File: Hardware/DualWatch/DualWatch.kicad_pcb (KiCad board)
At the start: 4 copper layers, 41.2 x 42.1 mm, 154 parts, among them J1 NFC, J2 NRF_Debug, J3 USB_C_Receptacle_USB2.0, J4 Conn_01x02_Pin, Q1 BSS123, Q2 IRLM2803, U1 NRF5340-QKAA-R7, U10 SN74LV1T34DCK, U11 SN74LV1T34DCK, U12 SN74LV1T34DCK, U13 SN74LV1T34DCK, U14 SN74LV1T34DCK, U15 SN74LV1T34DCK, U16 SN74LV1T34DCK, U17 SN74LV1T34DCK, U18 SN74LV1T34DCK, U20 NPM1100-QDAA-R7, U21 TPS63030DSK, U22 TPS63030DSK, U23 SN74LV1T34DCK, U24 SN74LV1T34DCK, U3 74LVC1G3157, U4 NRF7002-QFAA-R, U5 DPX165950DT-8126A1, U7 LIS3DH, U8 SN74LV1T34DCK, Y1 32.768kHz, Y2 32MHz, Y3 40Mhz

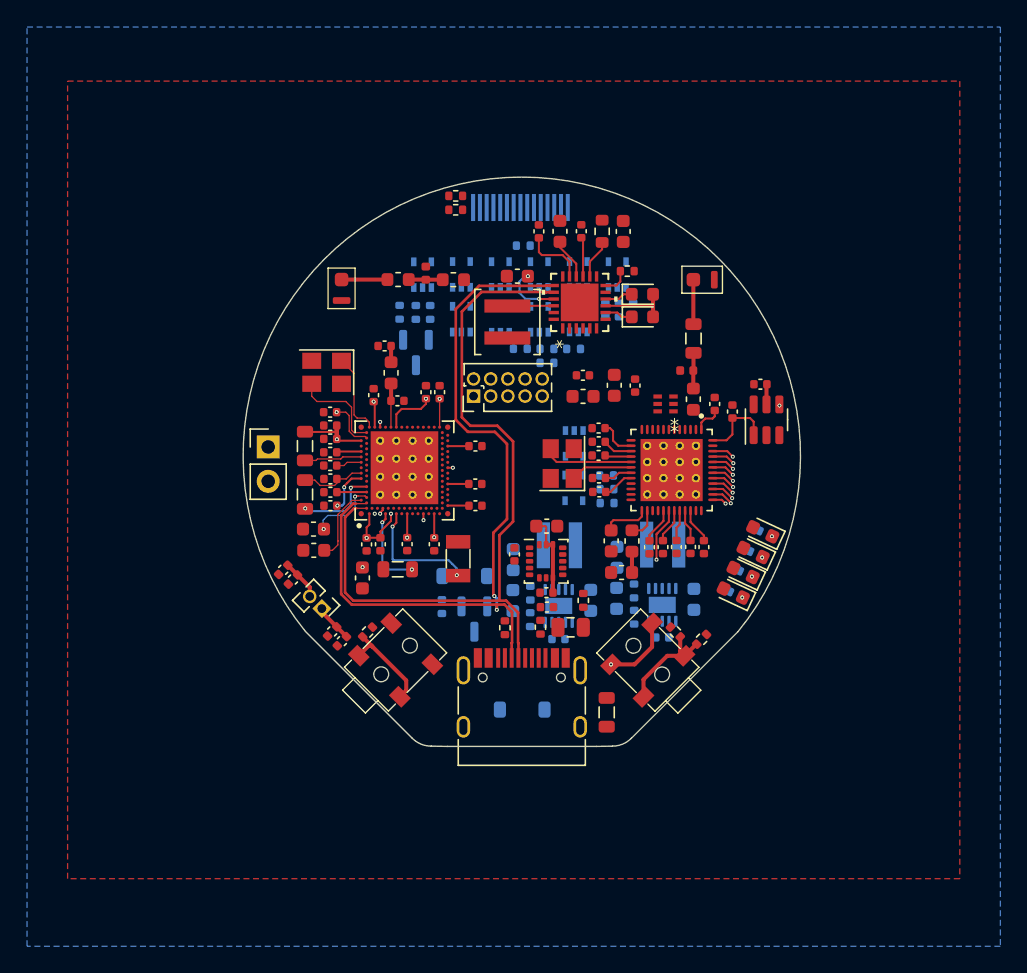
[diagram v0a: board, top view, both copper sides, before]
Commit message: update pcb
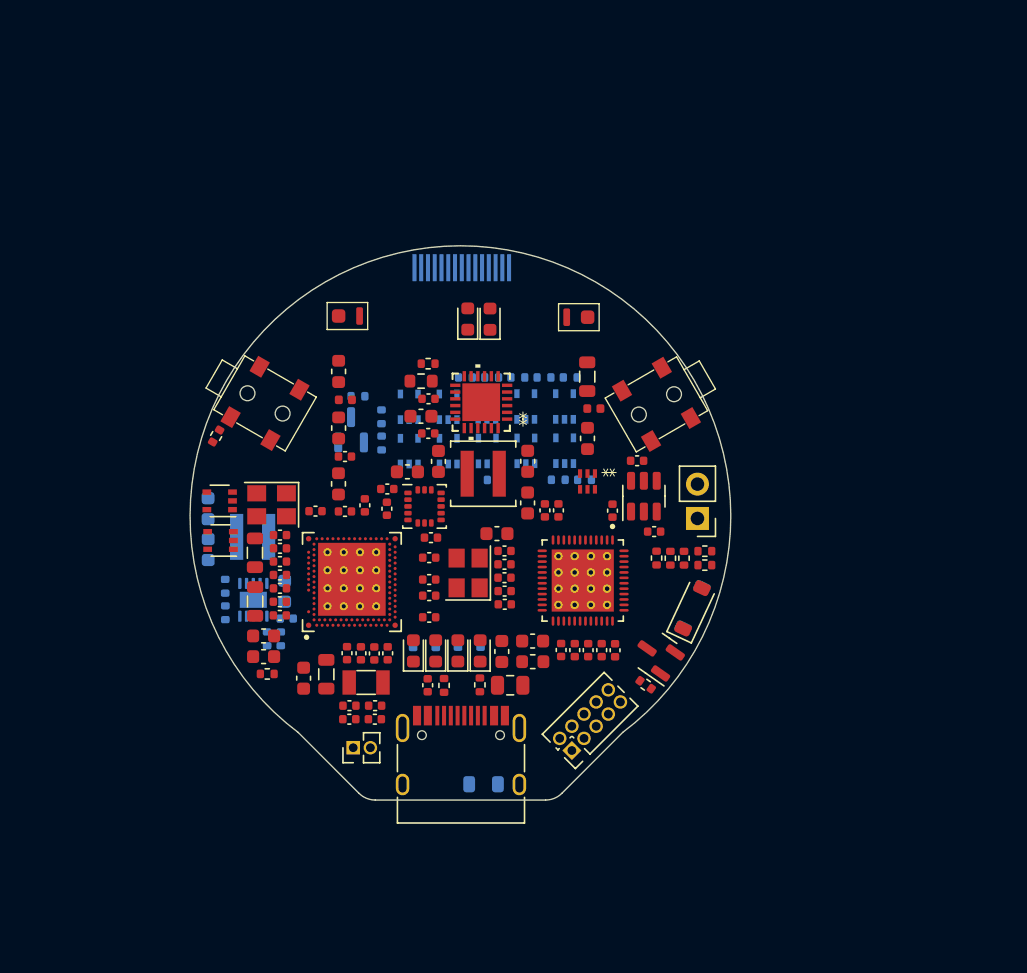
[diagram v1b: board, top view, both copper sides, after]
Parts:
- removed C60, C61, C62, C63: 10uF, Capacitor_SMD:C_0603_1608Metric
- removed L15: 1.5uH, Inductor_SMD:L_Coilcraft_XAL4020-XXX
- removed R31: 100R, Resistor_SMD:R_0402_1005Metric
- removed R32: 10K, Resistor_SMD:R_0402_1005Metric
- removed U23, U24: SN74LV1T34DCK, Package_TO_SOT_SMD:SOT-353_SC-70-5
- added U9: SN74LV1T34DCK, Package_TO_SOT_SMD:SOT-353_SC-70-5, B.Cu at (139.2, 90.4)
- C59: value 100nF -> 10uF; footprint Capacitor_SMD:C_0402_1005Metric -> Capacitor_SMD:C_0603_1608Metric
- D4, Q2, R18: moved to F.Cu
- L8: moved to B.Cu
- R21: value 100K -> 178K
- R22: value 178K -> 1M
- R23: value 261K -> 1K; moved to F.Cu
- R24: value 1M -> 10K; moved to F.Cu
- R25: value 1K -> 10K
- R26: value 10K -> 100R; moved to B.Cu
- R27: value 10K -> 100R
- R30: value 100R -> 10K; moved to F.Cu
- U18: value SN74LV1T34DCK -> ~; footprint Package_TO_SOT_SMD:SOT-353_SC-70-5 -> 1-28-LCD-Touch:1.28LCD-TP
- U19: value ~ -> NPM1100-QDAA-R7; footprint 1-28-LCD-Touch:1.28LCD-TP -> NPM1100-QDAA-R7:QFN24_NPM1100_NOR; moved to F.Cu
- U20: value NPM1100-QDAA-R7 -> TPS63030DSK; footprint NPM1100-QDAA-R7:QFN24_NPM1100_NOR -> Package_SON:WSON-10-1EP_2.5x2.5mm_P0.5mm_EP1.2x2mm; moved to B.Cu
- U21, U22: value TPS63030DSK -> SN74LV1T34DCK; footprint Package_SON:WSON-10-1EP_2.5x2.5mm_P0.5mm_EP1.2x2mm -> Package_TO_SOT_SMD:SOT-353_SC-70-5; moved to F.Cu
- moved R30 40.5 mm to (122.0, 89.3), turned to 60 degrees
- moved C58 36.1 mm to (121.4, 97.7)
- moved C59 34.9 mm to (121.4, 94.6), turned to 90 degrees
- moved U22 33.6 mm to (122.2, 94.1), turned to 180 degrees
- moved U20 32.7 mm to (124.7, 101.4), turned to -90 degrees
- moved J4 32.2 mm to (157.6, 95.4), turned to 180 degrees
- moved R15 32.1 mm to (158.1, 97.8), turned to 0 degrees
- moved R16 32.1 mm to (158.1, 98.8), turned to 180 degrees
- moved R22 30.3 mm to (122.7, 100.4)
- moved R19 27.5 mm to (125.8, 104.3), turned to 90 degrees
- moved D5 27.3 mm to (136.6, 105.1), turned to 90 degrees
- moved J2 27.2 mm to (148.3, 112.5), turned to 135 degrees
- moved R20 27.0 mm to (126.8, 104.3), turned to -90 degrees
- moved R29 26.4 mm to (136.6, 105.4), turned to 90 degrees
- moved U21 25.5 mm to (122.3, 97.0), turned to 180 degrees
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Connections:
- C54 pad 2: Net-(U20-DEC) -> Net-(U19-DEC)
- C57 pad 2: Net-(U21-PS/SYNC) -> Net-(U20-PS/SYNC)
- C58 pad 1: VIN -> +3V3
- C59 pad 1: GND -> +3V3
- C59 pad 2: Net-(U22-PS/SYNC) -> GND
- L13 pad 1: Net-(U20-SW) -> Net-(U19-SW)
- L14 pad 1: Net-(U21-L2) -> Net-(U20-L2)
- L14 pad 2: Net-(U21-L1) -> Net-(U20-L1)
- R17 pad 1: Net-(U20-ICHG) -> Net-(U19-ICHG)
- R21 pad 2: Net-(U21-FB) -> Net-(U20-FB)
- R22 pad 1: GND -> Net-(U20-FB)
- R22 pad 2: Net-(U22-FB) -> +3V3
- R23 pad 1: Net-(U21-FB) -> /DC DC/BTN
- R23 pad 2: +1V8 -> Net-(D4-A)
- R24 pad 1: Net-(U22-FB) -> Net-(D4-A)
- R24 pad 2: +3V3 -> GND
- R25 pad 1: /DC DC/BTN -> /DC DC/REG_EN
- R25 pad 2: Net-(D4-A) -> GND
- R26 pad 1: Net-(D4-A) -> Net-(D8-K)
- R27 pad 1: /DC DC/REG_EN -> Net-(D6-K)
- R28 pad 1: Net-(D8-K) -> Net-(D7-K)
- R29 pad 1: Net-(D6-K) -> Net-(D5-K)
- R30 pad 1: Net-(D7-K) -> +1V8
- R30 pad 2: GND -> /MCU/P1.13
- TH1 pad 1: Net-(U20-NTC) -> Net-(U19-NTC)
- U10 pad 2: /LCD/SPI_SCK -> /LCD/SPI_CS
- U10 pad 4: /LCD/SCK -> /LCD/CS
- U11 pad 2: /LCD/SPI_CS -> /LCD/LCD_DC
- U11 pad 4: /LCD/CS -> /LCD/DC
- U12 pad 2: /LCD/LCD_DC -> /LCD/LCD_RESET
- U12 pad 4: /LCD/DC -> /LCD/LCD_RST
- U13 pad 2: /LCD/LCD_RESET -> /LCD/LCD_BL
- U13 pad 4: /LCD/LCD_RST -> /LCD/BL
- U14 pad 2: /LCD/LCD_BL -> /LCD/I2C_SDA
- U14 pad 4: /LCD/BL -> /LCD/SDA
- U15 pad 2: /LCD/I2C_SDA -> /LCD/I2C_SCL
- U15 pad 4: /LCD/SDA -> /LCD/SCL
- U16 pad 2: /LCD/I2C_SCL -> /LCD/TP_RESET
- U16 pad 4: /LCD/SCL -> /LCD/TP_RST
- U17 pad 2: /LCD/TP_RESET -> /LCD/TP_INT
- U17 pad 4: /LCD/TP_RST -> /LCD/INT
- U18 pad 1: unconnected-(U18-NC-Pad1) -> GND
- U18 pad 2: /LCD/TP_INT -> /LCD/LEDK
- U18 pad 3: GND -> +3V3
- U18 pad 4: /LCD/INT -> +3V3
- U18 pad 5: +3V3 -> /LCD/DC
- U19 pad 1: GND -> +1V8
- U19 pad 10: +3V3 -> /MCU/P1.07
- U19 pad 11: GND -> /MCU/P1.09
- U19 pad 12: /LCD/TP_RST -> Net-(U19-ICHG)
- U19 pad 13: /LCD/INT -> unconnected-(U19-NC-Pad13)
- U19 pad 14: /LCD/SDA -> Net-(U19-NTC)
- U19 pad 15: /LCD/SCL -> /DC DC/VBAT
- U19 pad 2: /LCD/LEDK -> GND
- U19 pad 3: +3V3 -> GND
- U19 pad 4: +3V3 -> unconnected-(U19-NC-Pad4)
- U19 pad 5: /LCD/DC -> /nPM1100/VSYS
- U19 pad 6: /LCD/CS -> /MCU/P1.10
- U19 pad 7: /LCD/SCK -> /MCU/P1.08
- U19 pad 8: /LCD/MOSI -> /MCU/P1.06
- U19 pad 9: /LCD/LCD_RST -> /nPM1100/VSYS
- U20 pad 1: +1V8 -> +3V3
- U20 pad 10: /MCU/P1.07 -> Net-(U20-FB)
- U20 pad 11: /MCU/P1.09 -> GND
- U20 pad 2: GND -> Net-(U20-L2)
- U20 pad 4: unconnected-(U20-NC-Pad4) -> Net-(U20-L1)
- U20 pad 5: /MCU/P1.05 -> VIN
- U20 pad 6: /MCU/P1.10 -> /DC DC/REG_EN
- U20 pad 7: /MCU/P1.08 -> Net-(U20-PS/SYNC)
- U20 pad 8: /MCU/P1.06 -> Net-(U20-PS/SYNC)
- U20 pad 9: /nPM1100/VSYS -> GND
- U21 pad 1: +1V8 -> unconnected-(U21-NC-Pad1)
- U21 pad 2: Net-(U21-L2) -> /DC DC/REG_ENABLE
- U21 pad 4: Net-(U21-L1) -> /DC DC/REG_EN
- U21 pad 5: VIN -> +3V3
- U22 pad 1: +3V3 -> unconnected-(U22-NC-Pad1)
- U22 pad 2: Net-(U22-L2) -> /DC DC/BTN
- U22 pad 4: Net-(U22-L1) -> /DC DC/WAKE_UP
- U22 pad 5: VIN -> +1V8
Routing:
- net /MCU/USB_D-: track 58.5 -> 0.00 mm, vias 2 -> 0
- net /MCU/USB_D+: track 56.2 -> 0.00 mm
- net +1V8: track 29.9 -> 0.00 mm, vias 11 -> 0
- net +3V3: track 16.0 -> 0.00 mm, vias 2 -> 0
- net Net-(U1A-DECR): track 10.3 -> 0.00 mm, vias 2 -> 0
- net /MCU/XL1: track 9.02 -> 0.00 mm, vias 2 -> 0
- net /nPM1100/VSYS: track 8.88 -> 0.00 mm
- net /DC DC/VBAT: track 8.24 -> 0.00 mm, vias 1 -> 0
- net Net-(D4-A): track 7.84 -> 0.00 mm
- net /MCU/P1.13: track 7.48 -> 0.00 mm
- net /MCU/XC2: track 7.09 -> 0.00 mm
- net /WIFI/XOP: track 6.67 -> 0.00 mm
- net Net-(U1A-DCCH): track 6.16 -> 0.00 mm, vias 2 -> 0
- net Net-(U1A-DCCD): track 6.13 -> 0.00 mm, vias 2 -> 0
- net /MCU/XC1: track 6.11 -> 0.00 mm
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- removed copper zone on In2.Cu, net +1V8
- removed copper zone on B.Cu, net GND
- removed copper zone on F.Cu, net GND
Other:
- board size 41.2 x 42.1 mm -> 40 x 41 mm
